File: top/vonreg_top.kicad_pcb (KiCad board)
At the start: 2 copper layers, 110 x 91.9 mm, 17 parts, among them K1 SW_Push, K10 SW_Push, K11 SW_Push, K12 SW_Push, K15 SW_Push, K2 SW_Push, K3 SW_Push, K4 SW_Push, K5 SW_Push, K6 SW_Push, K7 SW_Push, K8 SW_Push, K9 SW_Push

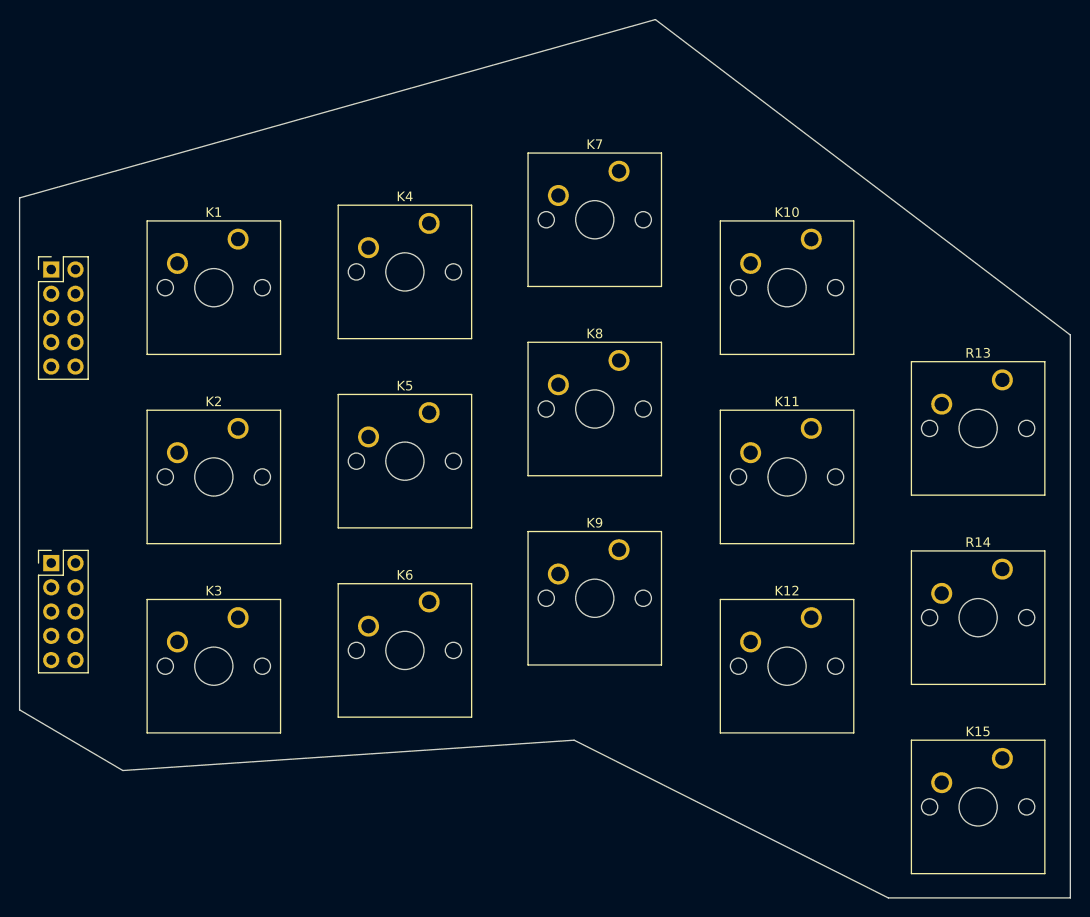
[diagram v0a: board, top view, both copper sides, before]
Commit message: Routing done, hopefully
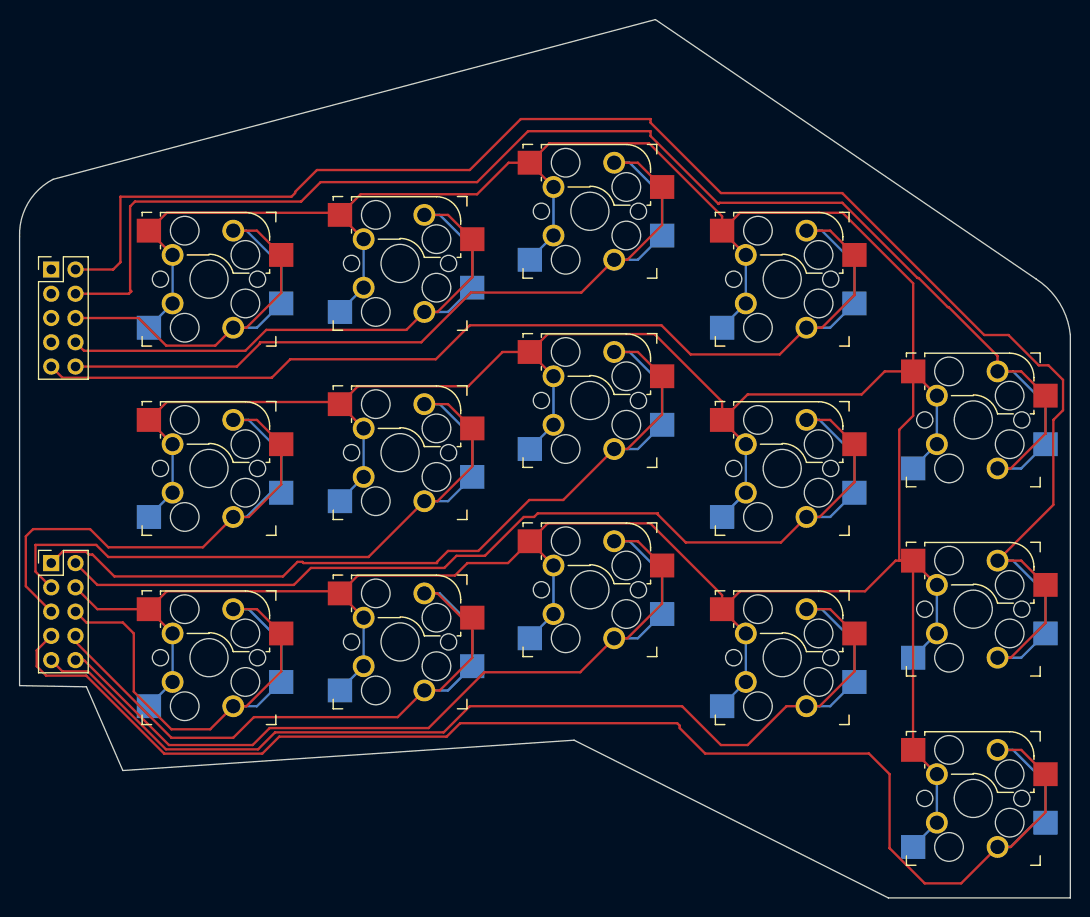
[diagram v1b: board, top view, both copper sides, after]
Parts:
- K1, K10, K11, K12, K15, K2, K3, K4, K5, K6, K7, K8, K9, R13, R14: footprint Button_Switch_Keyboard:SW_Cherry_MX_1.00u_PCB -> Button_Switch_Keyboard:Kailh_socket_MX_optional_reversible
- moved PinsTopA1 30.7 mm to (67.8, 59.4)
- moved PinsTopB1 30.7 mm to (67.8, 90.2)
- moved K11 5.18 mm to (144.3, 80.3)
- moved K15 5.18 mm to (164.3, 114.8)
- moved K2 5.18 mm to (84.3, 80.3)
- moved K4 5.18 mm to (104.3, 58.8)
- moved K5 5.18 mm to (104.3, 78.6)
- moved K6 5.18 mm to (104.3, 98.4)
- moved K7 5.18 mm to (124.2, 53.3)
- moved K8 5.18 mm to (124.2, 73.2)
- moved K9 5.18 mm to (124.2, 93.0)
- moved R13 5.18 mm to (164.3, 75.2)
- moved K1 5.18 mm to (84.3, 60.5)
- moved K10 5.18 mm to (144.3, 60.5)
- moved K12 5.18 mm to (144.3, 100.1)
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- gave numbers to parts that had none: 2
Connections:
- PinsTopA1 pad 1: /RT1 -> unconnected-(PinsTopA1-Pad1)
- PinsTopA1 pad 10: /RT10 -> /RT7
- PinsTopA1 pad 2: /RT2 -> /RT14
- PinsTopA1 pad 3: /RT3 -> unconnected-(PinsTopA1-Pad3)
- PinsTopA1 pad 4: /RT4 -> /RT13
- PinsTopA1 pad 5: /RT5 -> unconnected-(PinsTopA1-Pad5)
- PinsTopA1 pad 6: /RT6 -> /RT1
- PinsTopA1 pad 7: /RT7 -> unconnected-(PinsTopA1-Pad7)
- PinsTopA1 pad 8: /RT8 -> /RT4
- PinsTopA1 pad 9: /RT7 -> /RT10
- PinsTopB1 pad 1: /RT11 -> /RT8
- PinsTopB1 pad 10: GND -> /RT9
- PinsTopB1 pad 2: /RT12 -> /RT11
- PinsTopB1 pad 3: /RT13 -> /RT5
- PinsTopB1 pad 4: /RT14 -> GND
- PinsTopB1 pad 5: /RT15 -> /RT2
- PinsTopB1 pad 6: unconnected-(PinsTopB1-Pad6) -> /RT3
- PinsTopB1 pad 7: unconnected-(PinsTopB1-Pad7) -> /RT15
- PinsTopB1 pad 8: unconnected-(PinsTopB1-Pad8) -> /RT6
- PinsTopB1 pad 9: unconnected-(PinsTopB1-Pad9) -> /RT12
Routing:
- net GND: track 0.00 -> 515.2 mm
- net /RT14: track 0.00 -> 180.6 mm
- net /RT15: track 0.00 -> 156.0 mm
- net /RT13: track 0.00 -> 154.0 mm
- net /RT12: track 0.00 -> 121.5 mm
- net /RT10: track 0.00 -> 117.7 mm
- net /RT11: track 0.00 -> 116.2 mm
- net /RT8: track 0.00 -> 99.5 mm
- net /RT9: track 0.00 -> 98.0 mm
- net /RT7: track 0.00 -> 94.4 mm
- net /RT5: track 0.00 -> 82.1 mm
- net /RT6: track 0.00 -> 76.8 mm
- net /RT4: track 0.00 -> 71.9 mm
- net /RT2: track 0.00 -> 66.6 mm
- net /RT3: track 0.00 -> 59.5 mm
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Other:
- outline, holes or cut-outs redrawn
